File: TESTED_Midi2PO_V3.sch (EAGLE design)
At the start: 25 parts, among them IC1 TL071P, X1 PG203J

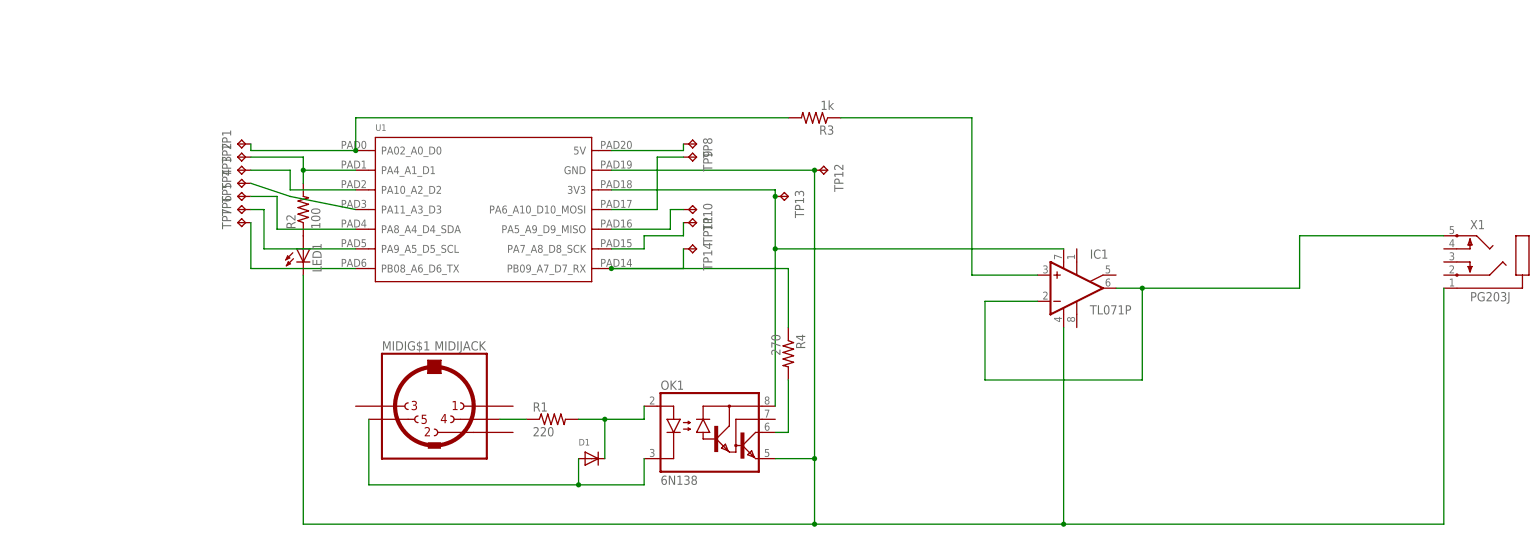
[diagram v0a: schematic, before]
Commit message: Restructured Project
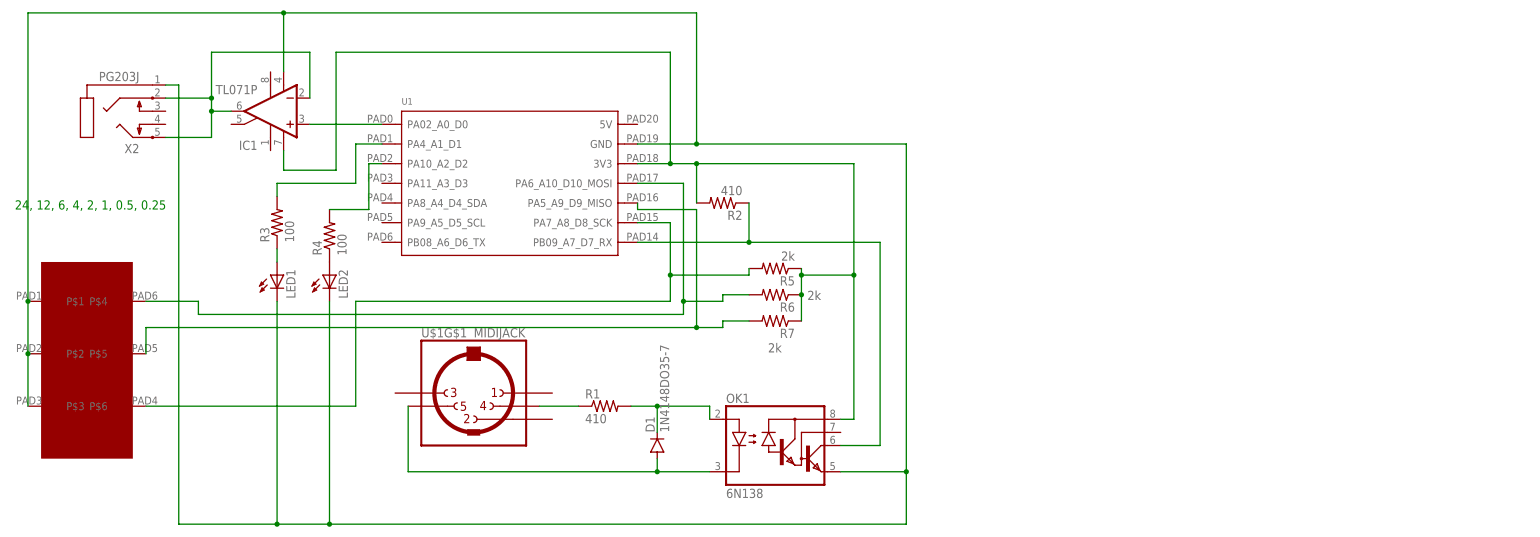
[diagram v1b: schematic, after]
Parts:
- removed MIDI: MIDIJACK, adafruit:MIDIJACK
- removed TP1, TP10, TP11, TP12, TP13, TP14, TP2, TP3, TP4, TP5, TP6, TP7, TP8, TP9: TPB2,54, testpad:TPB2,54
- removed X1: PG203J, con-hirschmann:PG203J
- added LED2: (no value), adafruit:LED5MM
- added R5, R6, R7: 2k, adafruit:R-US_0207/9
- added U$1: MIDIJACK, adafruit:MIDIJACK
- added U$2: MCNDA-03V, Vertical_DIP3_Sw:MCNDA-03V
- added X2: PG203J, con-hirschmann:PG203J
- D1: value (none) -> 1N4148DO35-7; device adafruit:DIODEDO-1N4148 -> diode:1N4148DO35-7
- IC1: device linear3:TL071P -> linear:TL071P
- LED1: device adafruit:LEDSFH480 -> adafruit:LED5MM; SPICEPREFIX (none) -> L
- R1: value 220 -> 410; device adafruit:R-US_0207/10 -> adafruit:R-US_0207/9
- R2: value 100 -> 410; device adafruit:R-US_0207/10 -> adafruit:R-US_0207/9
- R3: value 1k -> 100; device adafruit:R-US_0207/10 -> adafruit:R-US_0207/9; SPICEPREFIX (none) -> R
- R4: value 270 -> 100; device adafruit:R-US_0207/10 -> adafruit:R-US_0207/9
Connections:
- removed net N$10: IC1.+IN, R3.1
- removed net N$17: TP8.TP, U1.5V
- removed net N$18: TP9.TP, U1.PA6_A10_D10_MOSI
- removed net N$19: TP10.TP, U1.PA5_A9_D9_MISO
- removed net N$20: TP11.TP, U1.PA7_A8_D8_SCK
- removed net N$21: OK1.VO, R4.2
- net N$11: now also X2.2, X2.5; no longer X1.5
- net N$12: now also LED2.A, R4.1; no longer TP6.TP, U1.PA9_A5_D5_SCL
- net N$13: now also R4.2, U1.PA10_A2_D2; no longer TP7.TP, U1.PB08_A6_D6_TX
- net N$14: now also R7.2, U$2.P$5, U1.PA5_A9_D9_MISO; no longer LED1.A, R2.1
- net N$15: now also R5.2, U$2.P$6, U1.PA7_A8_D8_SCK; no longer IC1.V-, LED1.C, OK1.GND, TP12.TP, U1.GND, X1.1
- net N$16: now also IC1.V+, OK1.VCC, R5.1, R6.1, R7.1, U1.3V3; no longer TP2.TP, U1.PA4_A1_D1
- net N$2: now also U$1G$1.4; no longer MIDIG$1.4
- net N$3: now also U$1G$1.5; no longer MIDIG$1.5
- net N$4: now also IC1.V-, LED1.C, LED2.C, OK1.GND, U$2.P$1, U$2.P$2, U$2.P$3, U1.GND, X2.1; no longer TP3.TP, U1.PA10_A2_D2
- net N$5: now also OK1.VO, R2.1, U1.PB09_A7_D7_RX; no longer IC1.V+, OK1.VCC, TP13.TP, U1.3V3
- net N$6: now also R6.2, U$2.P$4, U1.PA6_A10_D10_MOSI; no longer R4.1, TP14.TP, U1.PB09_A7_D7_RX
- net N$7: now also IC1.+IN, U1.PA02_A0_D0; no longer TP4.TP, U1.PA11_A3_D3
- net N$8: now also LED1.A, R3.1; no longer R3.2, TP1.TP, U1.PA02_A0_D0
- net N$9: now also R3.2, U1.PA4_A1_D1; no longer TP5.TP, U1.PA8_A4_D4_SDA
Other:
- note added: "24, 12, 6, 4, 2, 1, 0.5, 0.25"
- moved on the sheet: IC1, LED1, OK1, R1, R2, R3, R4, U1
